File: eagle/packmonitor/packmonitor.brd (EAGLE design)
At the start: 61.8 x 18 mm, 28 parts, among them IC1 24C64, IC2 TCA4311A, IC3 AVRXDA32TQFP, IC4 ACS712

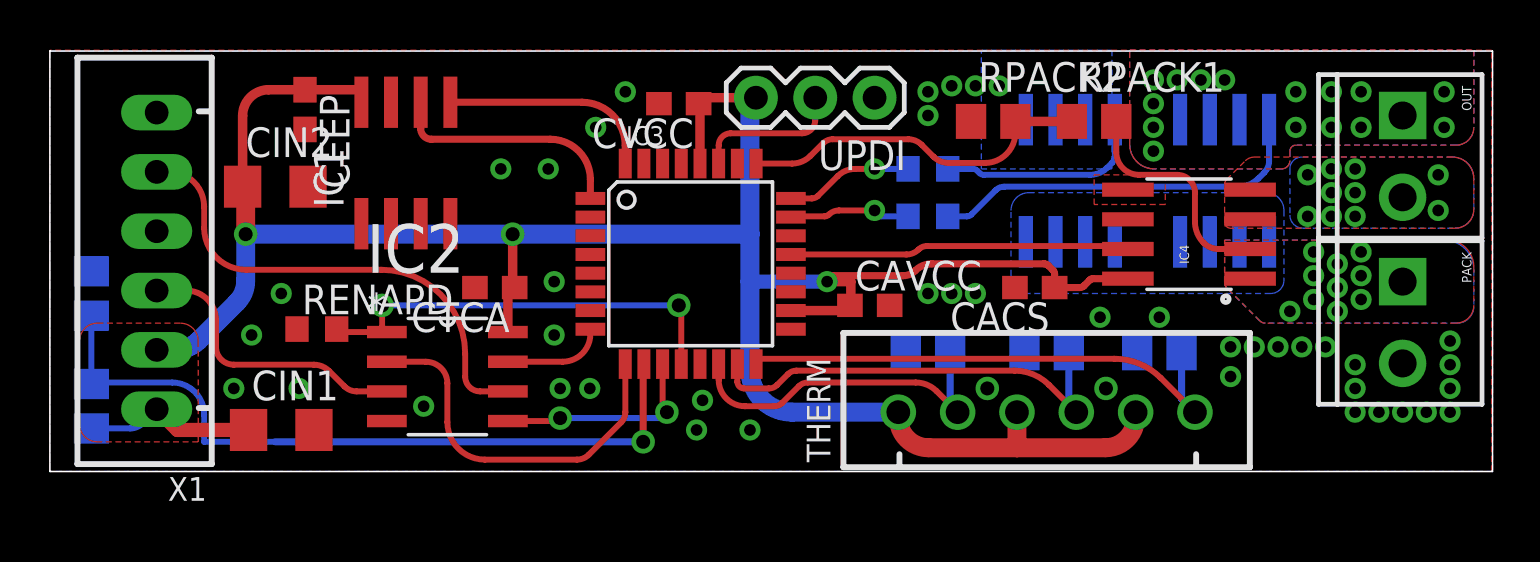
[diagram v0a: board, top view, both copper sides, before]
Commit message: final tweaks, fingers crossed order sent
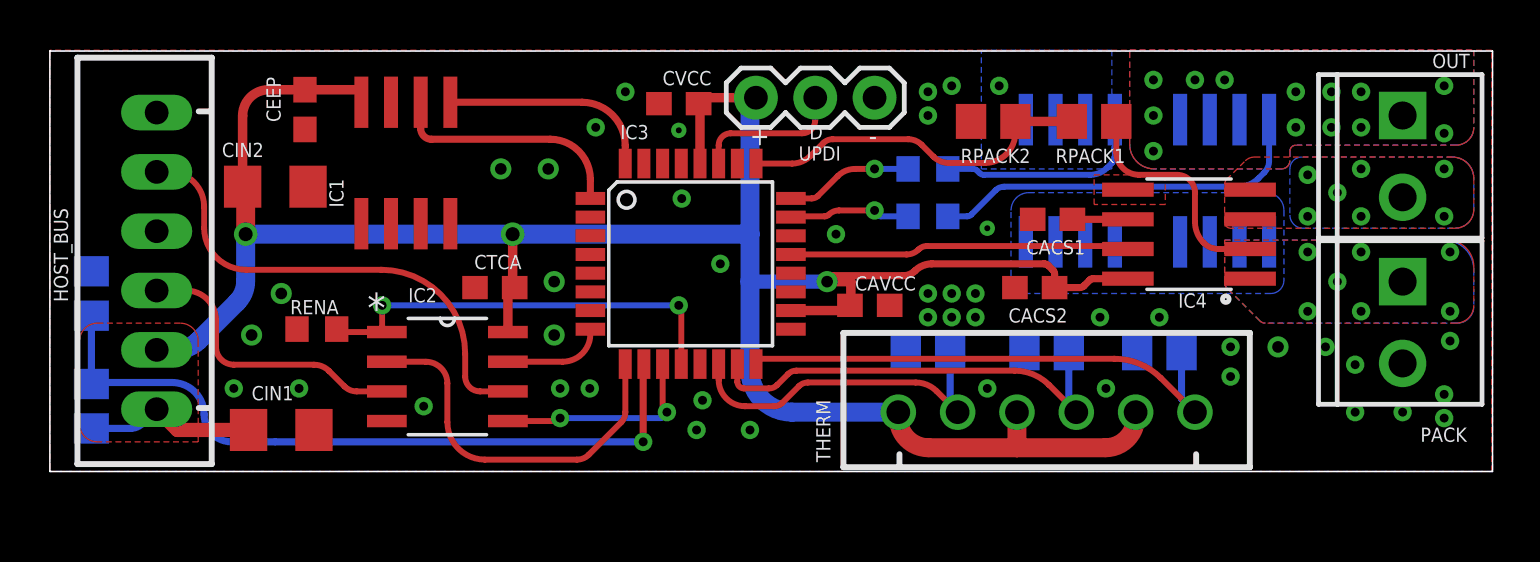
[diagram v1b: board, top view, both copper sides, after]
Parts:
- added CACS1: 1n, rcl:C0603
- renumbered CACS to CACS2, RENAPD to RENA, X1 to HOST_BUS
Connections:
- new net N$3: CACS1.1, IC4.6
- net GND: now also CACS1.2; no longer IC4.6
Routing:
- net N$3: track 0.00 -> 2.38 mm
- net VBUS: track 31.7 -> 31.0 mm
- net PACK+: vias 10 -> 7
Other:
- board text added: "(+)"
- board text added: "(-)"
- board text added: "+"
- board text added: "-"
- board text added: "D"
